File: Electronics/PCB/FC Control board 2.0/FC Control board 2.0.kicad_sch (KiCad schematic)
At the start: 85 parts, among them IC1 A3909GLNTR-T, IC2 A3909GLNTR-T, IC3 LTV-247, IC4 LTV-247, J1 USB_C_Receptacle_USB2.0, J2 CAM, J3 Servo, J4 Hall-M1, J5 Hall-M2, J6 Hall-M0, J7 Hall-M3, M0 Motor_DC_ALT, M1 Motor_DC_ALT, M2 Motor_DC_ALT, M3 Motor_DC_ALT, Q1 SQ2348ES-T1_BE3, SW1 RST, SW2 BOOT, U1 ESP32-S3-WROOM-1-N8, U2 AZ1117IH-3.3TRG1, U4 AZ1117D-5.0TRE1, U6 INA4181A3IPWR, U7 AZ1117IH-3.3TRG1, U8 LSM6DSM (LSM6DSMTR), U9 LM358_DFN

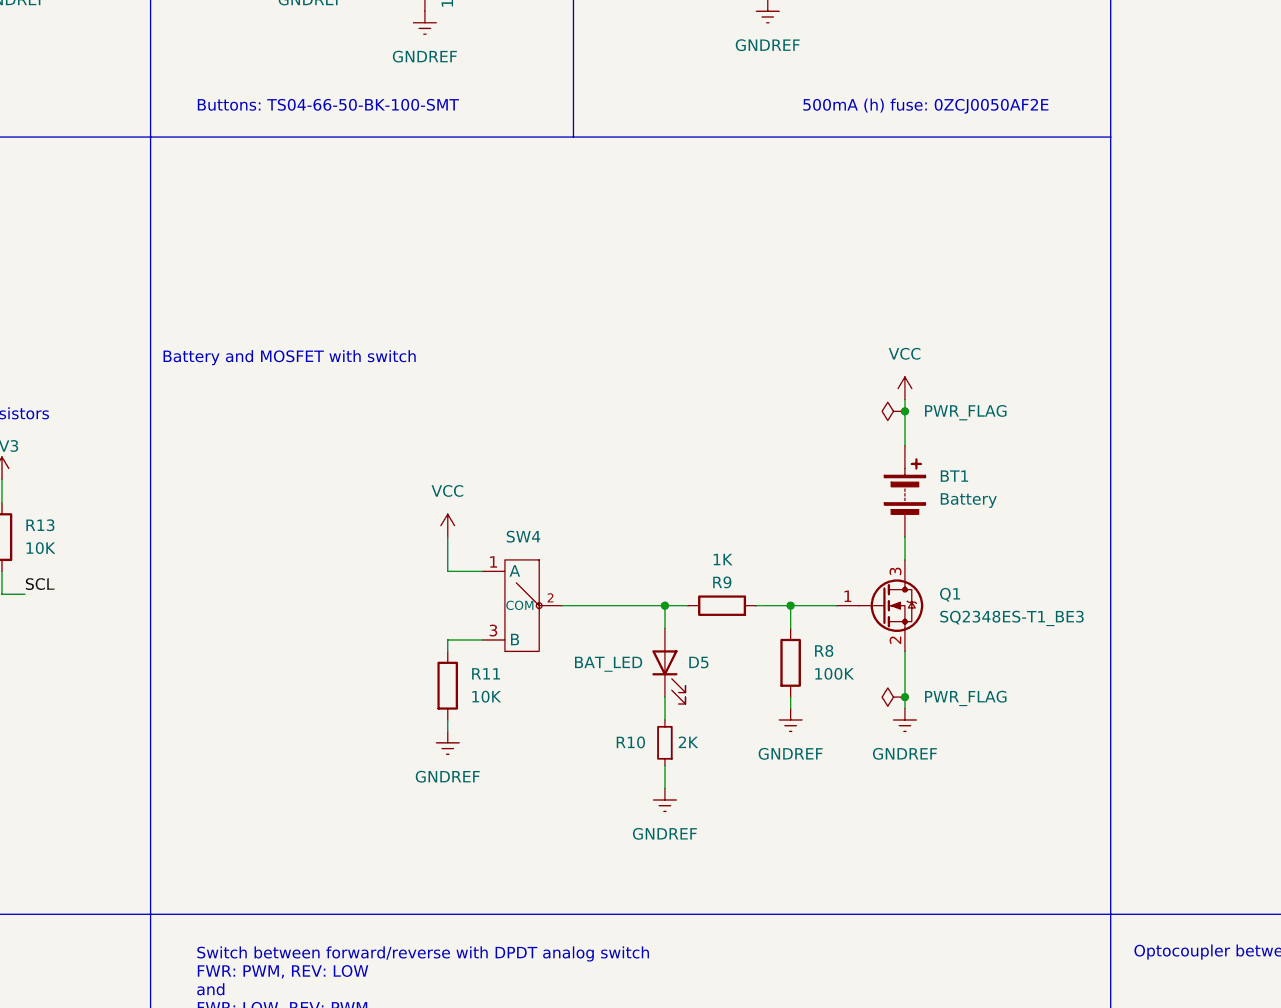
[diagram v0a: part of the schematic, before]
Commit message: Final version of 2.0 [Ordered]
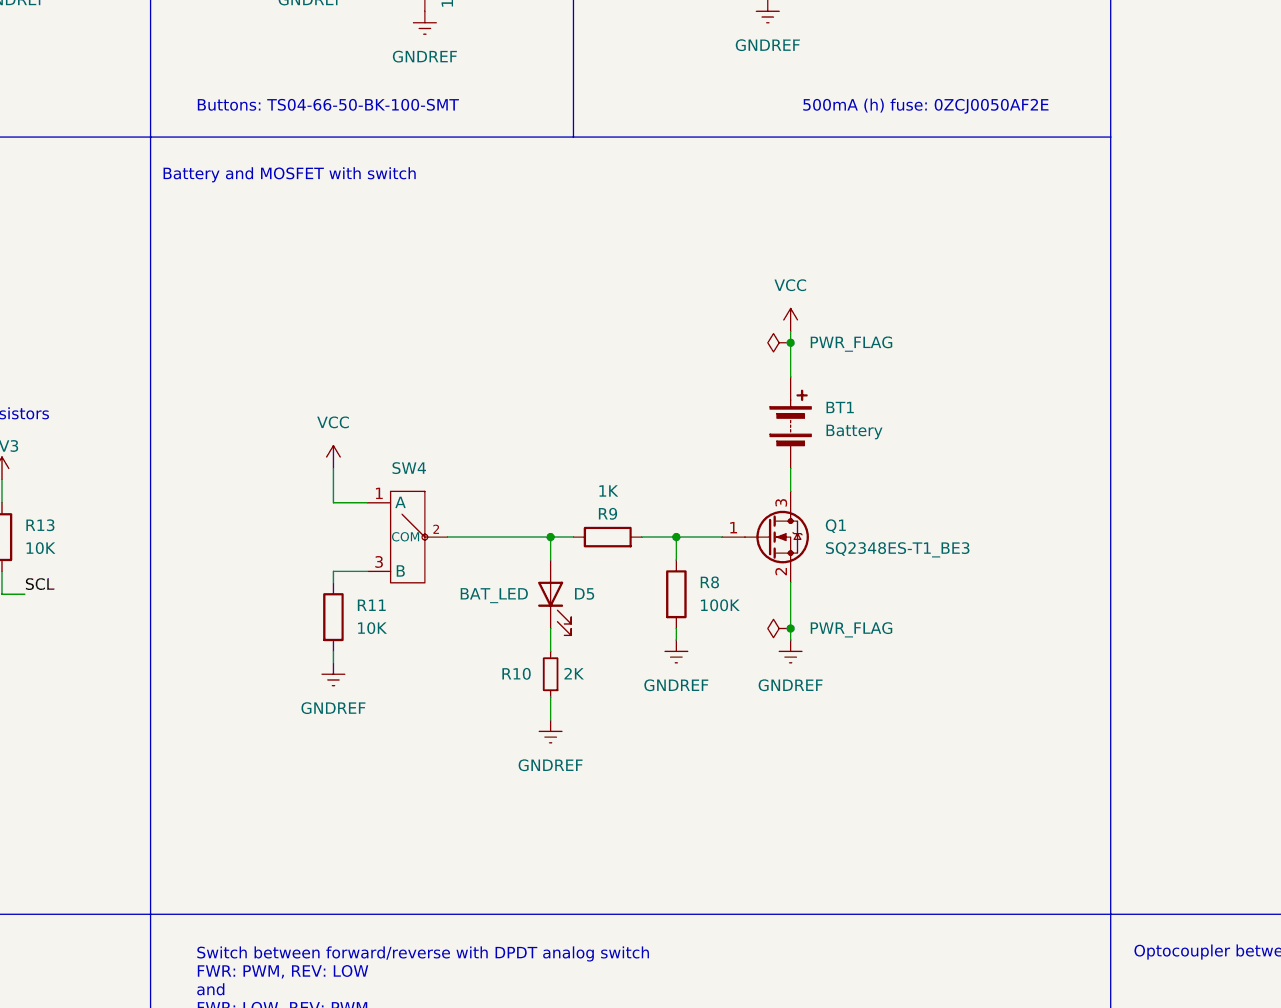
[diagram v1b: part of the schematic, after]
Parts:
- U9: footprint Package_DFN_QFN:DFN-8-1EP_2x2mm_P0.5mm_EP1.05x1.75mm -> Package_SO:SOIC-8-1EP_3.9x4.9mm_P1.27mm_EP2.514x3.2mm
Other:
- moved on the sheet: BT1, D5, Q1, R10, R11, R8, R9, SW4
